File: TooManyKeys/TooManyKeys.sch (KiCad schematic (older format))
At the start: 59 parts

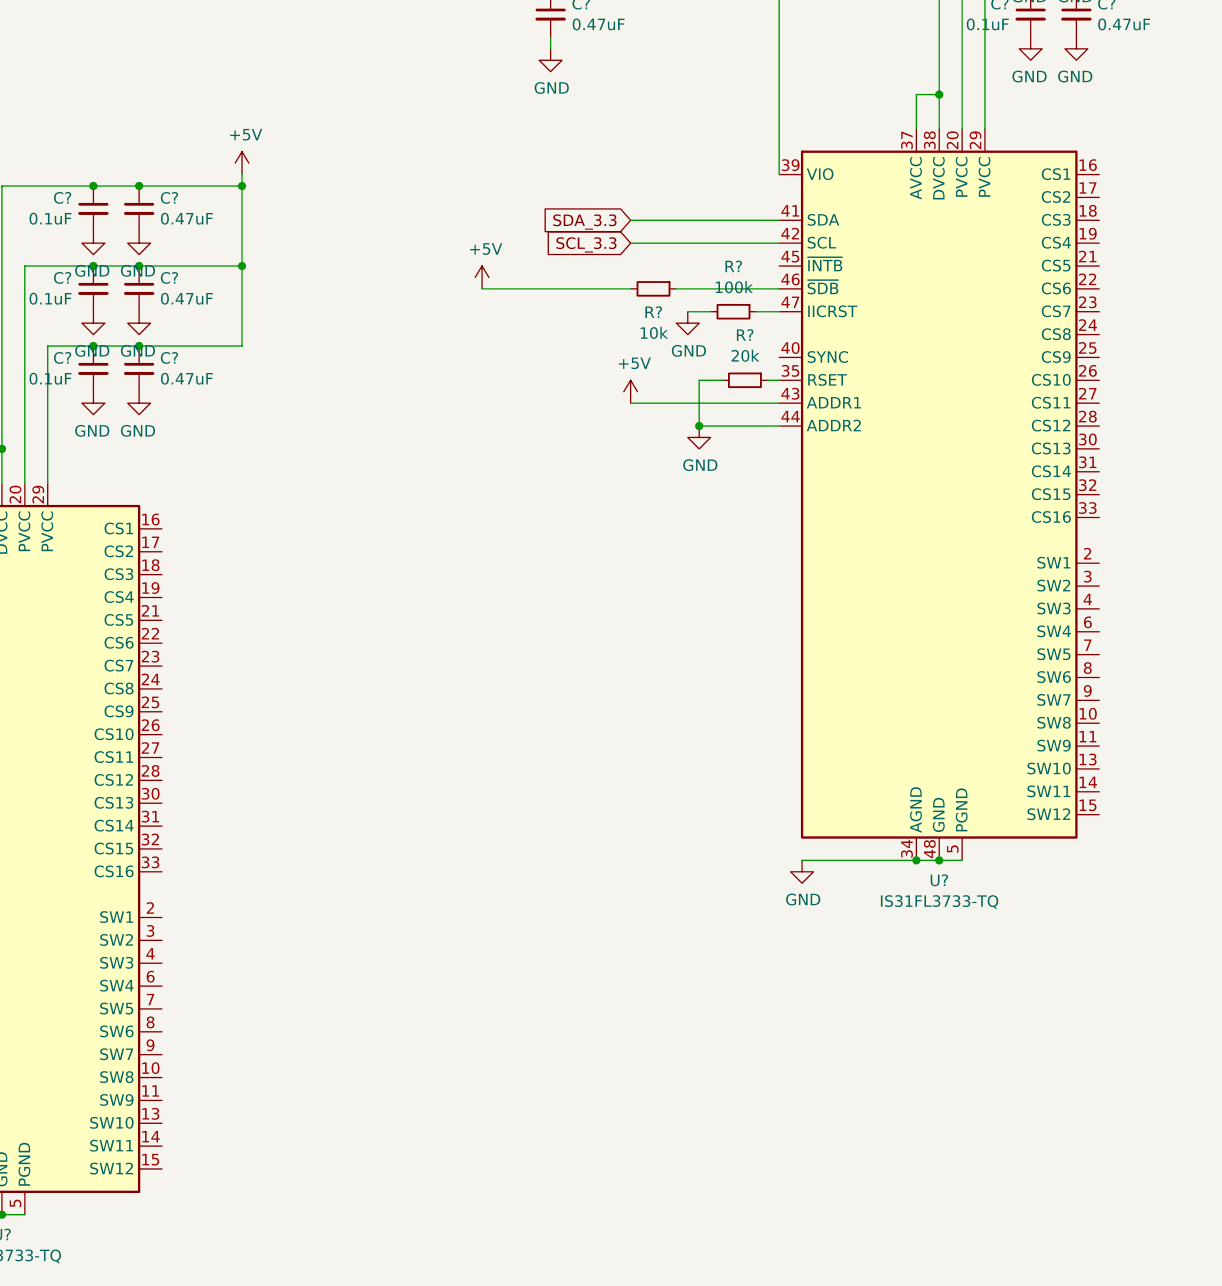
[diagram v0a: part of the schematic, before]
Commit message: V1 Schematics
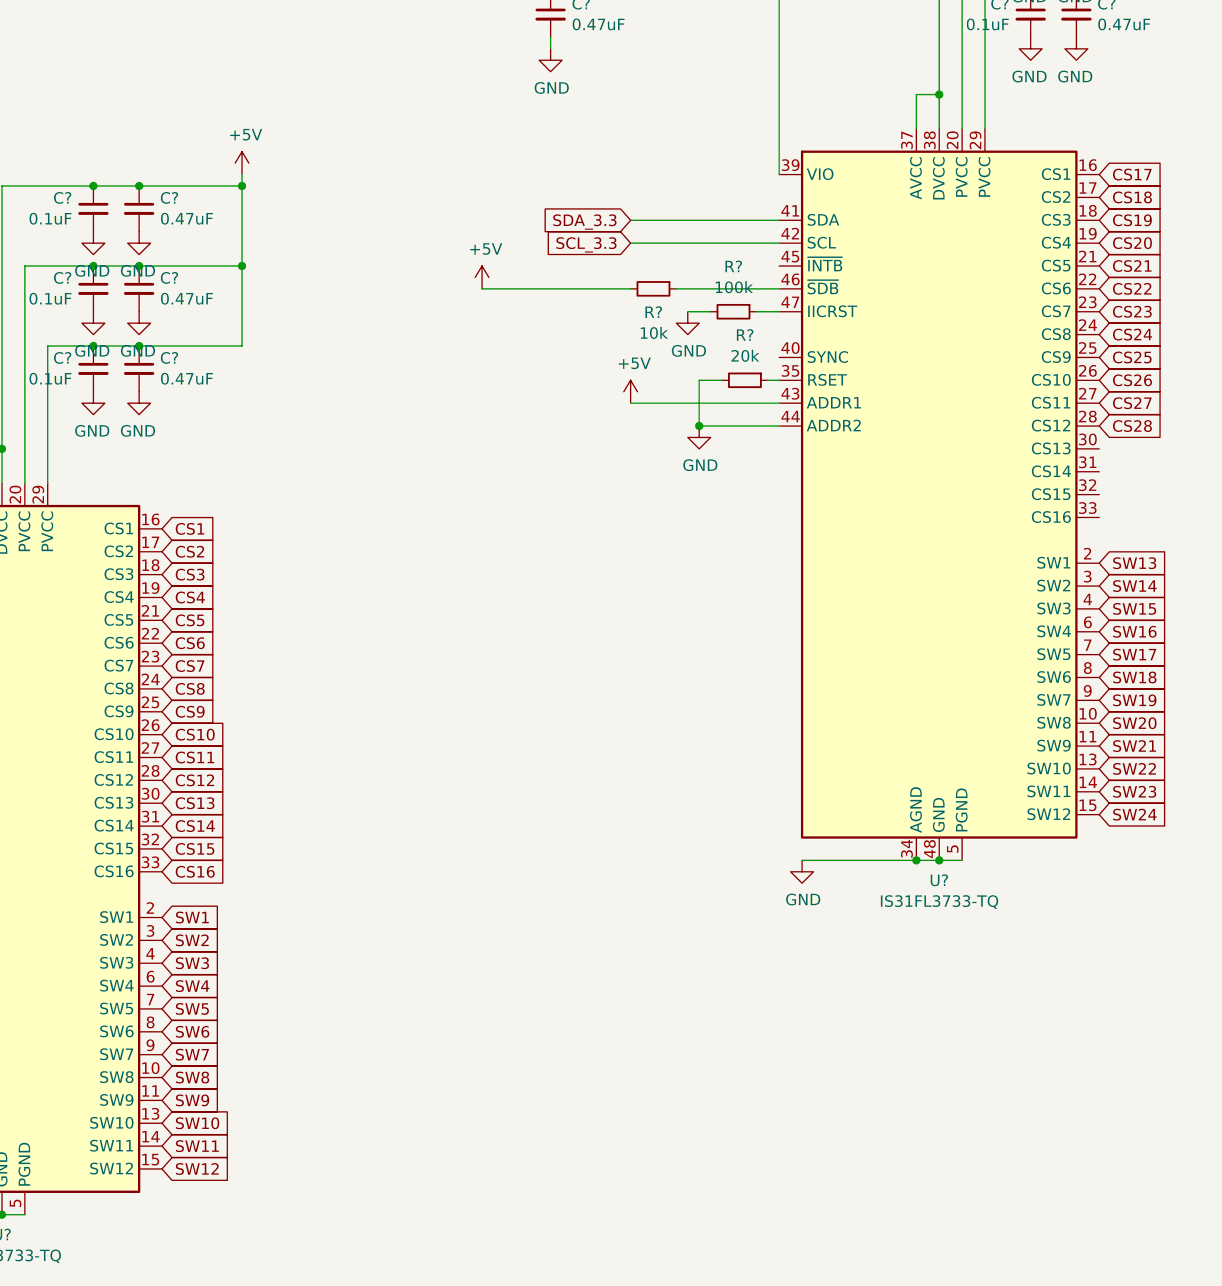
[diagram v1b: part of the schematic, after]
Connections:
- net SW8: now reaches MASTER_U?.10 (SW8)
- net SW9: now reaches MASTER_U?.11 (SW9)
- net SW10: now reaches MASTER_U?.13 (SW10)
- net SW11: now reaches MASTER_U?.14 (SW11)
- net SW12: now reaches MASTER_U?.15 (SW12)
- net CS1: now reaches MASTER_U?.16 (CS1)
- net CS2: now reaches MASTER_U?.17 (CS2)
- net CS3: now reaches MASTER_U?.18 (CS3)
- net CS4: now reaches MASTER_U?.19 (CS4)
- net SW1: now reaches MASTER_U?.2 (SW1)
- net CS5: now reaches MASTER_U?.21 (CS5)
- net CS6: now reaches MASTER_U?.22 (CS6)
- net CS7: now reaches MASTER_U?.23 (CS7)
- net CS8: now reaches MASTER_U?.24 (CS8)
- net CS9: now reaches MASTER_U?.25 (CS9)
- net CS10: now reaches MASTER_U?.26 (CS10)
- net CS11: now reaches MASTER_U?.27 (CS11)
- net CS12: now reaches MASTER_U?.28 (CS12)
- net SW2: now reaches MASTER_U?.3 (SW2)
- net CS13: now reaches MASTER_U?.30 (CS13)
- net CS14: now reaches MASTER_U?.31 (CS14)
- net CS15: now reaches MASTER_U?.32 (CS15)
- net CS16: now reaches MASTER_U?.33 (CS16)
- net SW3: now reaches MASTER_U?.4 (SW3)
- net SW4: now reaches MASTER_U?.6 (SW4)
- net SW5: now reaches MASTER_U?.7 (SW5)
- net SW6: now reaches MASTER_U?.8 (SW6)
- net SW7: now reaches MASTER_U?.9 (SW7)
- net SW20: now reaches SLAVE_U?.10 (SW8)
- net SW21: now reaches SLAVE_U?.11 (SW9)
- net SW22: now reaches SLAVE_U?.13 (SW10)
- net SW23: now reaches SLAVE_U?.14 (SW11)
- net SW24: now reaches SLAVE_U?.15 (SW12)
- net CS17: now reaches SLAVE_U?.16 (CS1)
- net CS18: now reaches SLAVE_U?.17 (CS2)
- net CS19: now reaches SLAVE_U?.18 (CS3)
- net CS20: now reaches SLAVE_U?.19 (CS4)
- net SW13: now reaches SLAVE_U?.2 (SW1)
- net CS21: now reaches SLAVE_U?.21 (CS5)
- net CS22: now reaches SLAVE_U?.22 (CS6)
- net CS23: now reaches SLAVE_U?.23 (CS7)
- net CS24: now reaches SLAVE_U?.24 (CS8)
- net CS25: now reaches SLAVE_U?.25 (CS9)
- net CS26: now reaches SLAVE_U?.26 (CS10)
- net CS27: now reaches SLAVE_U?.27 (CS11)
- net CS28: now reaches SLAVE_U?.28 (CS12)
- net SW14: now reaches SLAVE_U?.3 (SW2)
- net SW15: now reaches SLAVE_U?.4 (SW3)
- net SW16: now reaches SLAVE_U?.6 (SW4)
- net SW17: now reaches SLAVE_U?.7 (SW5)
- net SW18: now reaches SLAVE_U?.8 (SW6)
- net SW19: now reaches SLAVE_U?.9 (SW7)
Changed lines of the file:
@@
 Wire Wire Line
 	12550 5800 13200 5800
+Text GLabel 11150 8550 2    50   Input ~ 0
+SW1
+Text GLabel 11150 8650 2    50   Input ~ 0
+SW2
+Text GLabel 11150 8750 2    50   Input ~ 0
+SW3
+Text GLabel 11150 8850 2    50   Input ~ 0
+SW4
+Text GLabel 11150 8950 2    50   Input ~ 0
+SW5
+Text GLabel 11150 9050 2    50   Input ~ 0
+SW6
+Text GLabel 11150 9150 2    50   Input ~ 0
+SW7
+Text GLabel 11150 9250 2    50   Input ~ 0
+SW8
+Text GLabel 11150 9350 2    50   Input ~ 0
+SW9
+Text GLabel 11150 9450 2    50   Input ~ 0
+SW10
+Text GLabel 11150 9550 2    50   Input ~ 0
+SW11
+Text GLabel 11150 9650 2    50   Input ~ 0
+SW12
+Text GLabel 15250 7000 2    50   Input ~ 0
+SW13
+Text GLabel 15250 7100 2    50   Input ~ 0
+SW14
+Text GLabel 15250 7200 2    50   Input ~ 0
+SW15
+Text GLabel 15250 7300 2    50   Input ~ 0
+SW16
+Text GLabel 15250 7400 2    50   Input ~ 0
+SW17
+Text GLabel 15250 7500 2    50   Input ~ 0
+SW18
+Text GLabel 15250 7600 2    50   Input ~ 0
+SW19
+Text GLabel 15250 7700 2    50   Input ~ 0
+SW20
+Text GLabel 15250 7800 2    50   Input ~ 0
+SW21
+Text GLabel 15250 7900 2    50   Input ~ 0
+SW22
+Text GLabel 15250 8000 2    50   Input ~ 0
+SW23
+Text GLabel 15250 8100 2    50   Input ~ 0
+SW24
+Text GLabel 11150 6850 2    50   Input ~ 0
+CS1
+Text GLabel 11150 6950 2    50   Input ~ 0
+CS2
+Text GLabel 11150 7050 2    50   Input ~ 0
+CS3
+Text GLabel 11150 7150 2    50   Input ~ 0
+CS4
+Text GLabel 11150 7250 2    50   Input ~ 0
+CS5
+Text GLabel 11150 7350 2    50   Input ~ 0
+CS6
+Text GLabel 11150 7450 2    50   Input ~ 0
+CS7
+Text GLabel 11150 7550 2    50   Input ~ 0
+CS8
+Text GLabel 11150 7650 2    50   Input ~ 0
+CS9
+Text GLabel 11150 7750 2    50   Input ~ 0
+CS10
+Text GLabel 11150 7850 2    50   Input ~ 0
+CS11
+Text GLabel 11150 7950 2    50   Input ~ 0
+CS12
+Text GLabel 11150 8050 2    50   Input ~ 0
+CS13
+Text GLabel 11150 8150 2    50   Input ~ 0
+CS14
+Text GLabel 11150 8250 2    50   Input ~ 0
+CS15
+Text GLabel 11150 8350 2    50   Input ~ 0
+CS16
+Text GLabel 15250 5300 2    50   Input ~ 0
+CS17
+Text GLabel 15250 5400 2    50   Input ~ 0
+CS18
+Text GLabel 15250 5500 2    50   Input ~ 0
+CS19
+Text GLabel 15250 5600 2    50   Input ~ 0
+CS20
+Text GLabel 15250 5700 2    50   Input ~ 0
+CS21
+Text GLabel 15250 5800 2    50   Input ~ 0
+CS22
+Text GLabel 15250 5900 2    50   Input ~ 0
+CS23
+Text GLabel 15250 6000 2    50   Input ~ 0
+CS24
+Text GLabel 15250 6100 2    50   Input ~ 0
+CS25
+Text GLabel 15250 6200 2    50   Input ~ 0
+CS26
+Text GLabel 15250 6300 2    50   Input ~ 0
+CS27
+Text GLabel 15250 6400 2    50   Input ~ 0
+CS28
 $EndSCHEMATC
